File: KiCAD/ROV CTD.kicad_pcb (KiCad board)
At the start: 2 copper layers, 99.1 x 23.4 mm, 45 parts, among them J1 Conn_Coaxial, J10 1Wire1, J11 1Wire2, J12 1Wire3, J13 Interface, J14 Interface, J15 Conn_01x07_Pin, J6 Main In, M1 EZO-EC, M2 MS5803-14BA, U2 ATtiny1614-Arduino, U3 AP63205WU, U6 MAX3072E

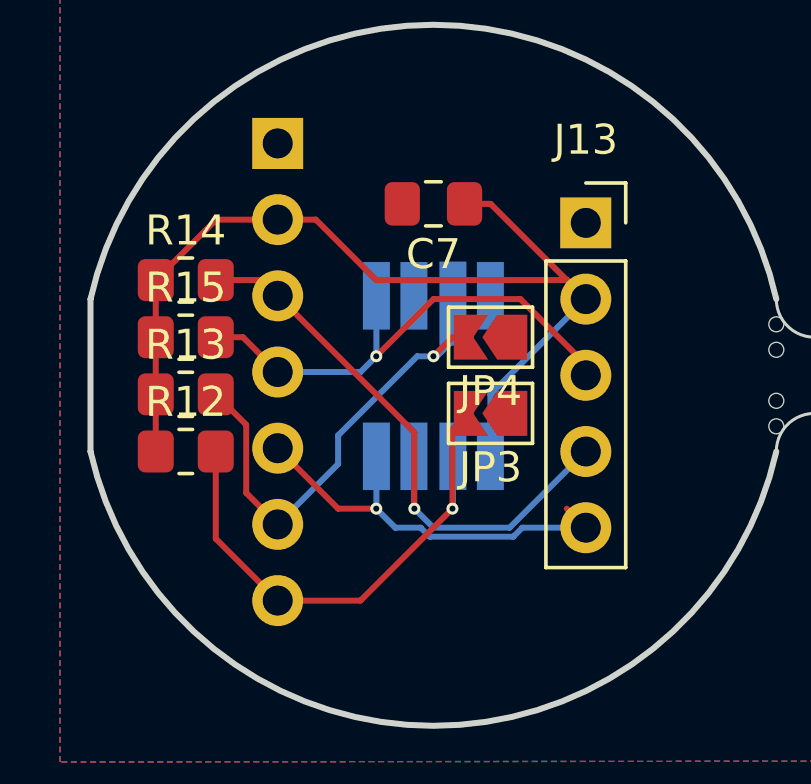
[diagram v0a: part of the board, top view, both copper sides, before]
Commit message: .
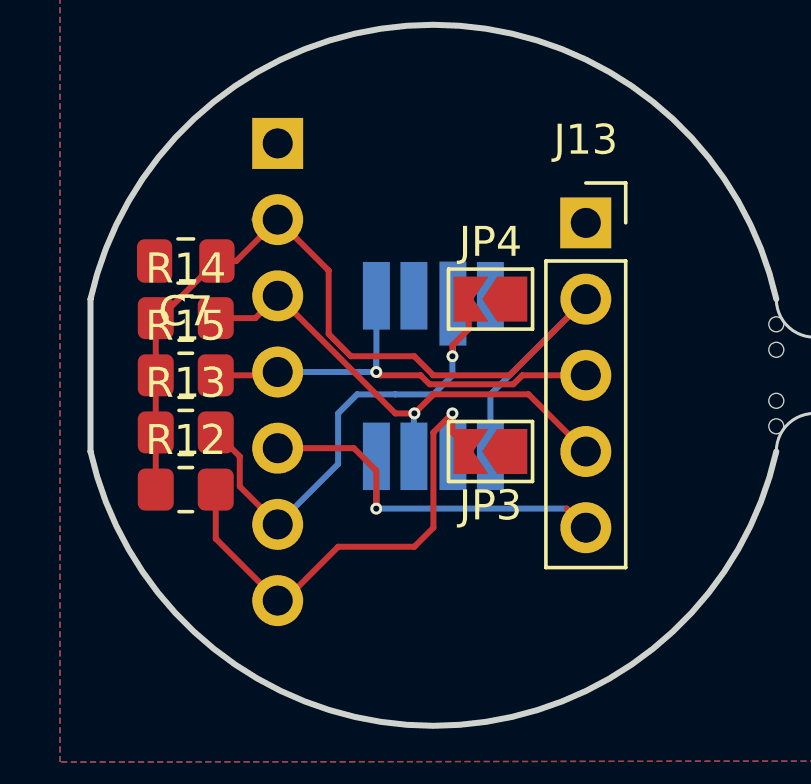
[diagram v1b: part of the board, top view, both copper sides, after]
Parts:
- moved C7 8.47 mm to (131.4, 72.4)
- moved JP4 1.27 mm to (141.6, 73.7)
- moved R12 1.27 mm to (131.4, 80.0)
- moved R13 1.27 mm to (131.4, 78.1)
- moved JP3 1.27 mm to (141.6, 78.7)
- moved R14 1.27 mm to (131.4, 74.3)
- moved R15 1.27 mm to (131.4, 76.2)
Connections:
- J14 pad 3: unconnected-(J14-Pin_3-Pad3) -> /SCL/SCLK
- J14 pad 4: unconnected-(J14-Pin_4-Pad4) -> /SDA/SDI
- J14 pad 5: unconnected-(J14-Pin_5-Pad5) -> /SDO
- M2 pad 4: unconnected-(M2-n/c-Pad4) -> (no net)
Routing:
- net /SDA/SDI: track 20.0 -> 16.8 mm
- net /SCL/SCLK: track 17.1 -> 15.2 mm
- net +3V3: track 34.9 -> 33.2 mm
- net /AD/CS: track 16.8 -> 17.3 mm
